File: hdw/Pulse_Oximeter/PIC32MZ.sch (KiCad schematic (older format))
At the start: 3 parts

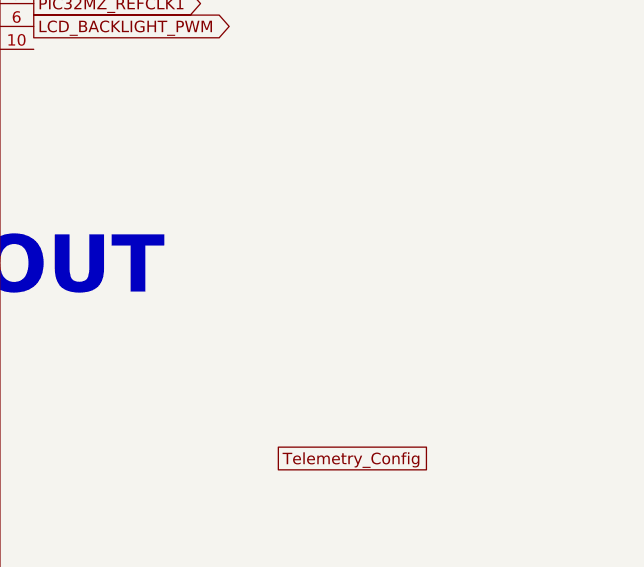
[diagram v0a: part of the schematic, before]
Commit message: Added SD card slot and backup RTC
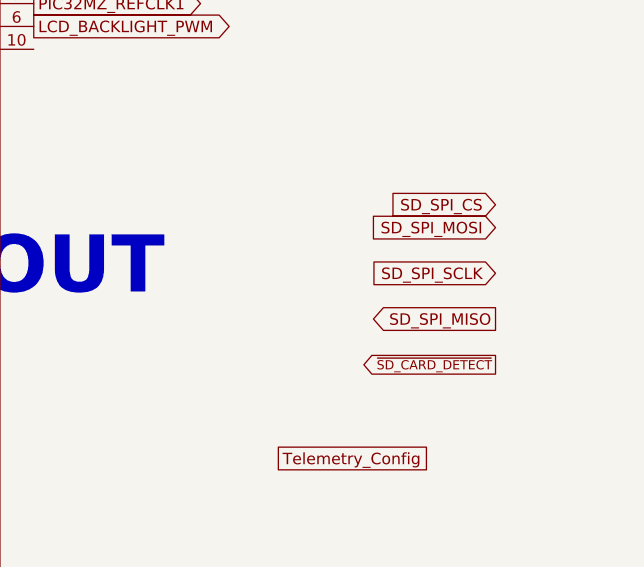
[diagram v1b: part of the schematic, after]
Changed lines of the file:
@@
 $Descr A 11000 8500
 encoding utf-8
-Sheet 11 20
+Sheet 11 22
 Title "Pulse Oximeter"
 Date "2019-04-11"
@@
 Text GLabel 8630 5200 2    50   UnSpc ~ 0
 Telemetry_Config
+Text GLabel 9580 4790 0    40   Output ~ 0
+~SD_CARD_DETECT
+Text GLabel 9580 4090 0    50   Input ~ 0
+SD_SPI_CS
+Text GLabel 9580 4190 0    50   Input ~ 0
+SD_SPI_MOSI
+Text GLabel 9580 4390 0    50   Input ~ 0
+SD_SPI_SCLK
+Text GLabel 9580 4590 0    50   Output ~ 0
+SD_SPI_MISO
 $EndSCHEMATC
